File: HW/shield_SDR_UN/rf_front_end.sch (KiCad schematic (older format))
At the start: 93 parts, among them Q1 MOSFET_P, U1 MAX5864, U2 MAX2830

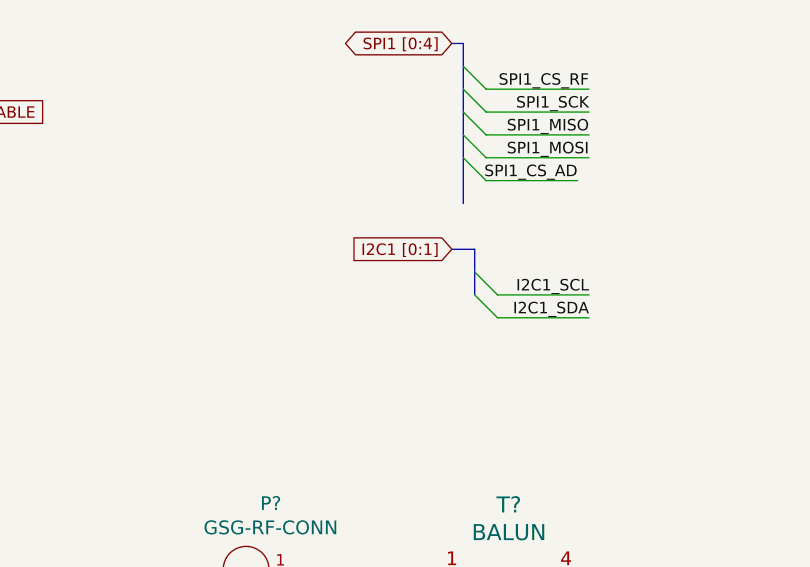
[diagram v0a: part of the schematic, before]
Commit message: i2c_complete
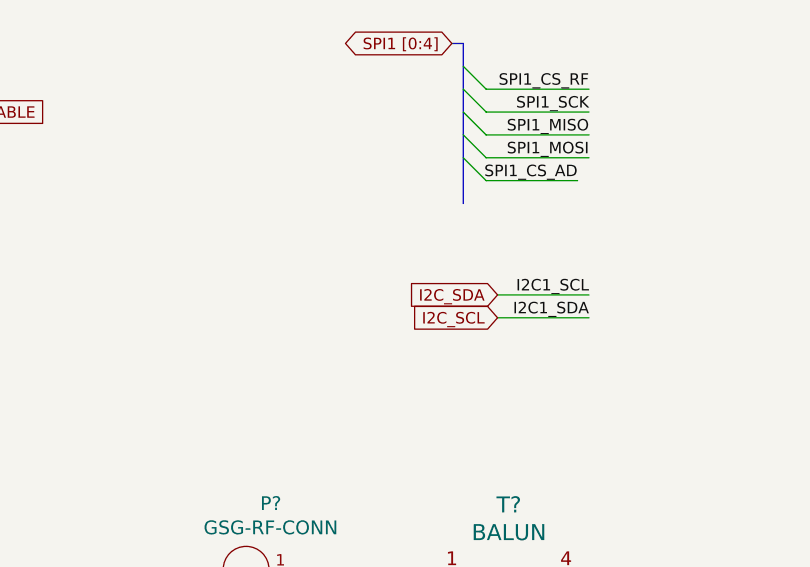
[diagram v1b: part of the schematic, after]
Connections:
- net I2C1_SCL renamed I2C_SDA
- net I2C1_SDA renamed I2C_SCL
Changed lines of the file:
@@
 Entry Wire Line
 	4300 1600 4400 1700
-Text Label 4850 2200 2    50   ~ 0
-I2C1_SCL
-Wire Wire Line
-	4450 2200 4850 2200
-Text Label 4850 2300 2    50   ~ 0
-I2C1_SDA
-Wire Wire Line
-	4450 2300 4850 2300
-Entry Wire Line
-	4350 2100 4450 2200
-Entry Wire Line
-	4350 2200 4450 2300
-Wire Bus Line
-	4350 2000 4250 2000
-Text GLabel 4250 2000 0    50   Input ~ 0
-I2C1 [0:1]
 Text Label 14750 3750 2    50   ~ 0
 SPI1_SCK
@@
 Text Notes 7350 6350 0    50   ~ 0
 MCU\n
-Wire Bus Line
-	4350 2000 4350 2200
+Wire Wire Line
+	4450 2300 4850 2300
+Text Label 4850 2300 2    50   ~ 0
+I2C1_SDA
+Wire Wire Line
+	4450 2200 4850 2200
+Text Label 4850 2200 2    50   ~ 0
+I2C1_SCL
+Text GLabel 4450 2300 0    50   Input ~ 0
+I2C_SCL
+Text GLabel 4450 2200 0    50   Input ~ 0
+I2C_SDA
 Wire Bus Line
 	4300 1100 4300 1800
